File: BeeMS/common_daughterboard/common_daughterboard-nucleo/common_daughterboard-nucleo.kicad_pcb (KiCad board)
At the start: 2 copper layers, 27 parts, among them J1 OUT_CONN, J2 TERM, J3 IN_CONN, J4 HEAD, J5 TAIL, J6 Conn_02x10_Odd_Even, Q1 BSS138, Q2 BSS138, U1 MCP2558FD-xSN

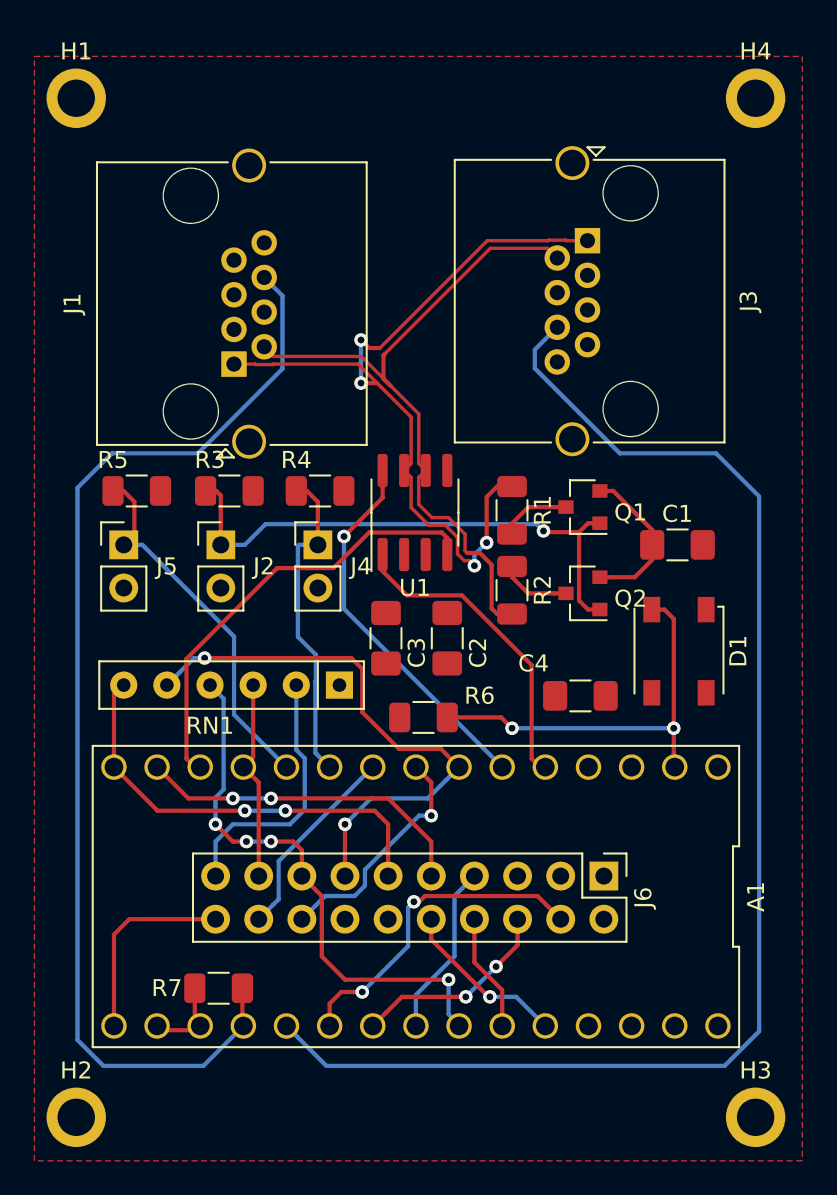
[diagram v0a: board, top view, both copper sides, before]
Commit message: BeeMS Common Daughterboard V0.0.1
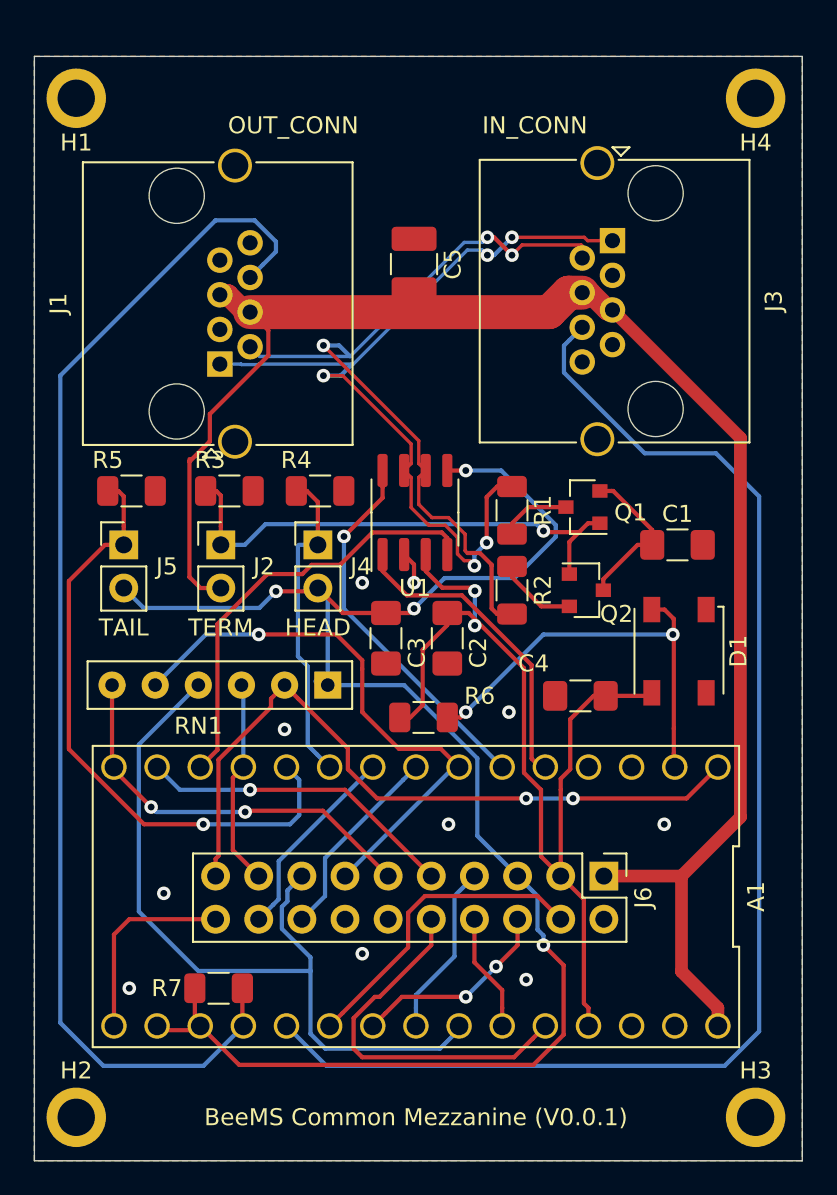
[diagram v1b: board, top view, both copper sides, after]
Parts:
- added C5: 47uF, Capacitor_SMD:C_1210_3225Metric_Pad1.42x2.65mm_HandSolder, F.Cu at (119.9, 109.8)
- added svg2mod: G***, BeeMS:Half-U-Half-car-thresh, B.Cu at (119.9, 111.3)
- moved J3 1.47 mm to (131.6, 108.4)
- moved J1 0.83 mm to (108.5, 115.7)
- moved RN1 0.69 mm to (114.8, 134.6)
- moved R5 0.31 mm to (103.3, 123.1)
- moved Q2 0.27 mm to (130.0, 129.0), turned to 0 degrees
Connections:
- Q2 pad 2: Net-(C1-Pad1) -> Net-(Q2-Pad2)
- Q2 pad 3: Net-(Q2-Pad3) -> Net-(C1-Pad1)
- R2 pad 1: Net-(Q2-Pad3) -> Net-(Q2-Pad2)
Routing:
- net +12V: track 0.00 -> 98.3 mm
- net +3V3: track 5.59 -> 101.6 mm, vias 0 -> 4
- net +5V: track 0.00 -> 57.8 mm, vias 0 -> 2
- net I2C2_SCL: track 15.6 -> 42.7 mm, vias 0 -> 2
- net I2C1_SCL: track 32.2 -> 46.6 mm, vias 4 -> 0
- net Net-(A1-Pad11): track 22.4 -> 36.7 mm, vias 0 -> 1
- net A3: track 10.0 -> 21.9 mm, vias 1 -> 0
- net CAN_-: track 41.8 -> 48.3 mm, vias 0 -> 3
- net NBR_OUT: track 66.9 -> 72.9 mm
- net Net-(Q2-Pad2): track 0.00 -> 4.71 mm
- net Net-(Q2-Pad3): track 4.20 -> 0.00 mm
- net Net-(J2-Pad1): track 32.6 -> 29.9 mm
- net CAN_+: track 48.9 -> 51.3 mm, vias 4 -> 5
- net D0: track 13.9 -> 11.7 mm, vias 1 -> 0
- net GND: track 0.00 -> 1.90 mm, vias 0 -> 10
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- added copper zone on B.Cu, net GND
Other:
- board outline added: 45.2 x 65 mm
- board text added: "BeeMS Common Mezzanine (V0.0.1)"
